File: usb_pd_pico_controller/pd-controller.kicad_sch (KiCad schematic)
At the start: 15 parts, among them J5 USB_C_Receptacle_USB2.0_16P, Q1 STL6P3LLH6, U1 STUSB4531QTR

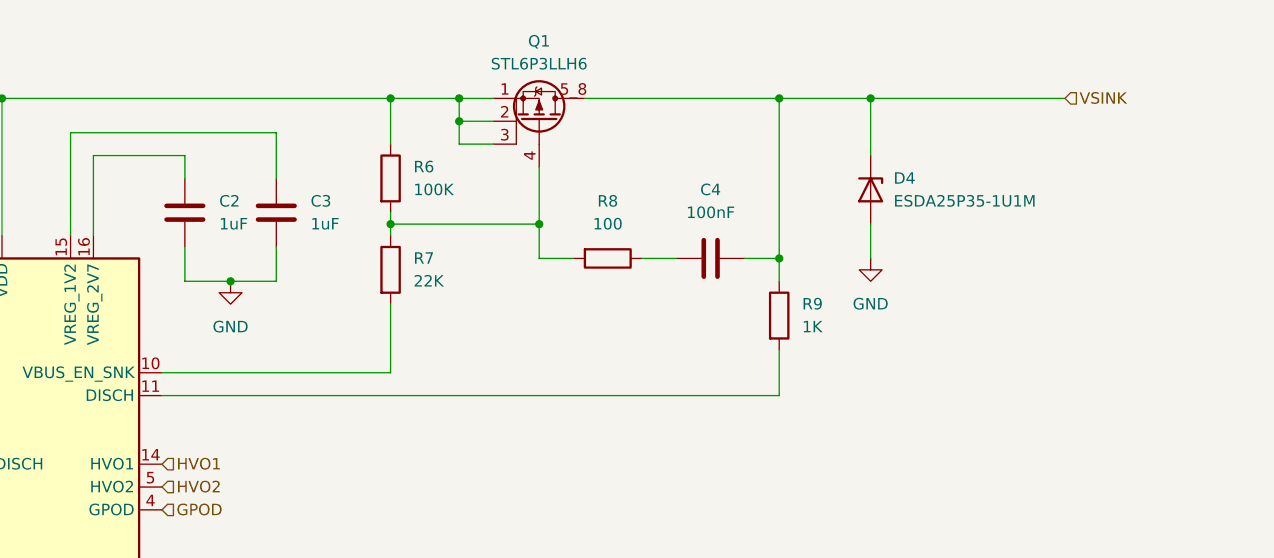
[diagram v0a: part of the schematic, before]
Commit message: Consolidated BOM item (100nF)
Signed-off-by: Thomas Flummer <tf@flummer.net>
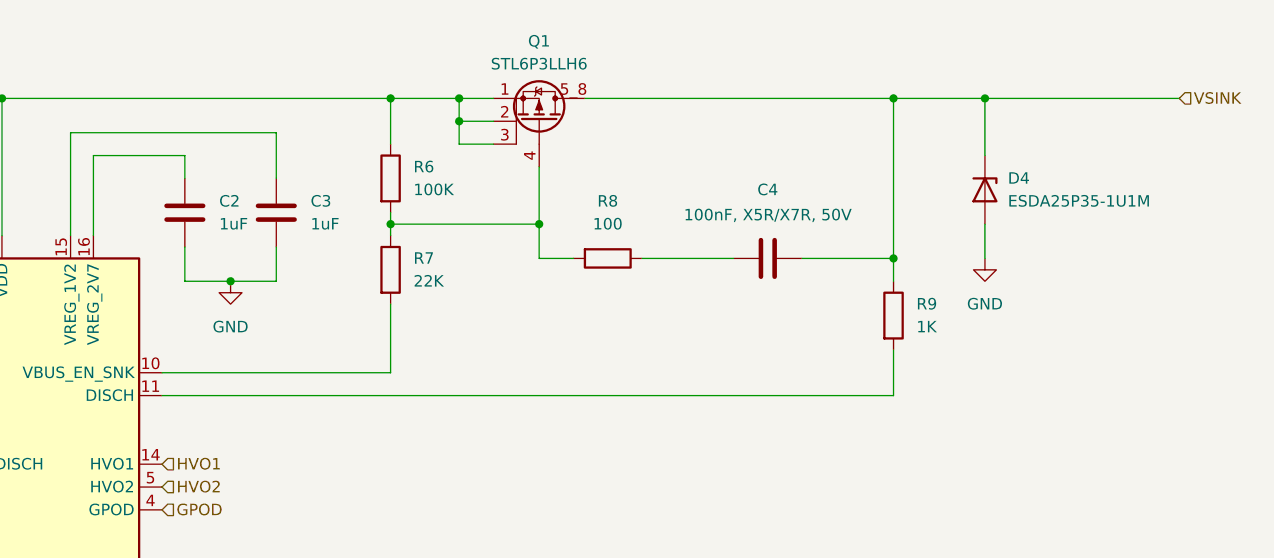
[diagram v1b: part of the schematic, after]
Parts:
- C4: value 100nF -> 100nF, X5R/X7R, 50V
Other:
- moved on the sheet: C4, D4, R9
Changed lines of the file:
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@@
-	)
-	(junction
-		(at 219.71 72.39)
-		(diameter 0)
-		(color 0 0 0 0)
 	)
 	(junction
@@
 	)
 	(junction
-		(at 219.71 54.61)
+		(at 232.41 54.61)
 		(diameter 0)
 		(color 0 0 0 0)
 	)
 	(junction
-		(at 229.87 54.61)
+		(at 242.57 54.61)
 		(diameter 0)
 		(color 0 0 0 0)
@@
 	)
 	(junction
+		(at 232.41 72.39)
+		(diameter 0)
+		(color 0 0 0 0)
+	)
+	(junction
 		(at 97.79 54.61)
 		(diameter 0)
@@
 	(wire
 		(pts
+			(xy 222.25 72.39) (xy 232.41 72.39)
+		)
+		(stroke
+			(width 0)
+			(type default)
+		)
+	)
+	(wire
+		(pts
 			(xy 50.8 54.61) (xy 73.66 54.61)
 		)
@@
 	(wire
 		(pts
-			(xy 198.12 54.61) (xy 219.71 54.61)
-		)
-		(stroke
-			(width 0)
-			(type default)
-		)
-	)
-	(wire
-		(pts
 			(xy 143.51 60.96) (xy 143.51 69.85)
 		)
@@
 	(wire
 		(pts
+			(xy 198.12 54.61) (xy 232.41 54.61)
+		)
+		(stroke
+			(width 0)
+			(type default)
+		)
+	)
+	(wire
+		(pts
 			(xy 68.58 82.55) (xy 68.58 59.69)
 		)
@@
 	(wire
 		(pts
-			(xy 204.47 72.39) (xy 208.28 72.39)
+			(xy 204.47 72.39) (xy 214.63 72.39)
 		)
 		(stroke
@@
 	(wire
 		(pts
-			(xy 219.71 72.39) (xy 219.71 54.61)
+			(xy 232.41 72.39) (xy 232.41 54.61)
 		)
 		(stroke
@@
 	(wire
 		(pts
-			(xy 219.71 82.55) (xy 219.71 87.63)
+			(xy 232.41 82.55) (xy 232.41 87.63)
 		)
 		(stroke
@@
 	(wire
 		(pts
-			(xy 229.87 68.58) (xy 229.87 72.39)
+			(xy 242.57 68.58) (xy 242.57 72.39)
 		)
 		(stroke
@@
 	(wire
 		(pts
-			(xy 215.9 72.39) (xy 219.71 72.39)
-		)
-		(stroke
-			(width 0)
-			(type default)
-		)
-	)
-	(wire
-		(pts
 			(xy 153.67 63.5) (xy 153.67 60.96)
 		)
@@
 	(wire
 		(pts
-			(xy 219.71 54.61) (xy 229.87 54.61)
-		)
-		(stroke
-			(width 0)
-			(type default)
-		)
-	)
-	(wire
-		(pts
-			(xy 219.71 72.39) (xy 219.71 74.93)
-		)
-		(stroke
-			(width 0)
-			(type default)
-		)
-	)
-	(wire
-		(pts
-			(xy 229.87 54.61) (xy 229.87 60.96)
+			(xy 232.41 54.61) (xy 242.57 54.61)
+		)
+		(stroke
+			(width 0)
+			(type default)
+		)
+	)
+	(wire
+		(pts
+			(xy 232.41 72.39) (xy 232.41 74.93)
+		)
+		(stroke
+			(width 0)
+			(type default)
+		)
+	)
+	(wire
+		(pts
+			(xy 151.13 87.63) (xy 232.41 87.63)
+		)
+		(stroke
+			(width 0)
+			(type default)
+		)
+	)
+	(wire
+		(pts
+			(xy 242.57 54.61) (xy 242.57 60.96)
 		)
 		(stroke
@@
 	(wire
 		(pts
-			(xy 219.71 87.63) (xy 151.13 87.63)
-		)
-		(stroke
-			(width 0)
-			(type default)
-		)
-	)
-	(wire
-		(pts
 			(xy 176.53 77.47) (xy 176.53 85.09)
 		)
@@
 	(wire
 		(pts
-			(xy 229.87 54.61) (xy 251.46 54.61)
+			(xy 242.57 54.61) (xy 264.16 54.61)
 		)
 		(stroke
@@
 	(hierarchical_label "VSINK"
 		(shape input)
-		(at 251.46 54.61 0)
+		(at 264.16 54.61 0)
 		(effects
 			(font
@@
 	(symbol
 		(lib_id "power:GND")
-		(at 229.87 72.39 0)
+		(at 242.57 72.39 0)
 		(unit 1)
 		(body_style 1)
@@
 		(fields_autoplaced yes)
 		(property "Reference" "#PWR018"
-			(at 229.87 78.74 0)
+			(at 242.57 78.74 0)
 			(hide yes)
 			(show_name no)
@@
 		)
 		(property "Value" "GND"
-			(at 229.87 77.47 0)
+			(at 242.57 77.47 0)
 			(show_name no)
 			(do_not_autoplace no)
@@
 		)
 		(property "Footprint" ""
-			(at 229.87 72.39 0)
+			(at 242.57 72.39 0)
 			(hide yes)
 			(show_name no)
@@
 		)
 		(property "Datasheet" ""
-			(at 229.87 72.39 0)
+			(at 242.57 72.39 0)
 			(hide yes)
 			(show_name no)
@@
 		)
 		(property "Description" "Power symbol creates a global label with name \"GND\" , ground"
-			(at 229.87 72.39 0)
+			(at 242.57 72.39 0)
 			(hide yes)
 			(show_name no)
@@
 	(symbol
 		(lib_id "Device:C")
-		(at 212.09 72.39 90)
+		(at 218.44 72.39 90)
 		(unit 1)
 		(body_style 1)
@@
 		(in_pos_files yes)
 		(dnp no)
-		(fields_autoplaced yes)
 		(property "Reference" "C4"
-			(at 212.09 64.77 90)
-			(show_name no)
-			(do_not_autoplace no)
-			(effects
-				(font
-					(size 1.27 1.27)
-				)
-			)
-		)
-		(property "Value" "100nF"
-			(at 212.09 67.31 90)
+			(at 218.44 64.77 90)
+			(show_name no)
+			(do_not_autoplace no)
+			(effects
+				(font
+					(size 1.27 1.27)
+				)
+			)
+		)
+		(property "Value" "100nF, X5R/X7R, 50V"
+			(at 218.44 67.564 90)
 			(show_name no)
 			(do_not_autoplace no)
@@
 		)
 		(property "Footprint" "Capacitor_SMD:C_0603_1608Metric"
-			(at 215.9 71.4248 0)
+			(at 222.25 71.4248 0)
 			(hide yes)
 			(show_name no)
@@
 		)
 		(property "Datasheet" ""
-			(at 212.09 72.39 0)
+			(at 218.44 72.39 0)
 			(hide yes)
 			(show_name no)
@@
 		)
 		(property "Description" "Unpolarized capacitor"
-			(at 212.09 72.39 0)
+			(at 218.44 72.39 0)
 			(hide yes)
 			(show_name no)
@@
 	(symbol
 		(lib_id "Device:R")
-		(at 219.71 78.74 0)
+		(at 232.41 78.74 0)
 		(unit 1)
 		(body_style 1)
@@
 		(fields_autoplaced yes)
 		(property "Reference" "R9"
-			(at 222.25 77.4699 0)
+			(at 234.95 77.4699 0)
 			(show_name no)
 			(do_not_autoplace no)
@@
 		)
 		(property "Value" "1K"
-			(at 222.25 80.0099 0)
+			(at 234.95 80.0099 0)
 			(show_name no)
 			(do_not_autoplace no)
@@
 		)
 		(property "Footprint" "Resistor_SMD:R_0603_1608Metric"
-			(at 217.932 78.74 90)
+			(at 230.632 78.74 90)
 			(hide yes)
 			(show_name no)
@@
 		)
 		(property "Datasheet" ""
-			(at 219.71 78.74 0)
+			(at 232.41 78.74 0)
 			(hide yes)
 			(show_name no)
@@
 		)
 		(property "Description" "Resistor"
-			(at 219.71 78.74 0)
+			(at 232.41 78.74 0)
 			(hide yes)
 			(show_name no)
@@
 	(symbol
 		(lib_id "Diode:ESD5Zxx")
-		(at 229.87 64.77 270)
+		(at 242.57 64.77 270)
 		(unit 1)
 		(body_style 1)
@@
 		(fields_autoplaced yes)
 		(property "Reference" "D4"
-			(at 232.41 63.4999 90)
+			(at 245.11 63.4999 90)
 			(show_name no)
 			(do_not_autoplace no)
@@
 		)
 		(property "Value" "ESDA25P35-1U1M"
-			(at 232.41 66.0399 90)
+			(at 245.11 66.0399 90)
 			(show_name no)
 			(do_not_autoplace no)
@@
 		)
 		(property "Footprint" "Diode_SMD:ST_QFN-2L_1.6x1.0mm"
-			(at 225.425 64.77 0)
+			(at 238.125 64.77 0)
 			(hide yes)
 			(show_name no)
@@
 		)
 		(property "Datasheet" "https://www.st.com/resource/en/datasheet/esda25p35-1u1m.pdf"
-			(at 229.87 64.77 0)
+			(at 242.57 64.77 0)
 			(hide yes)
 			(show_name no)
@@
 		)
 		(property "Description" "35 A - 8/20 us, 22 V TVS in QFN-2L"
-			(at 229.87 64.77 0)
-			(hide yes)
-			(show_name no)
+			(at 242.57 64.77 0)
+			(hide yes)
+			(show_name no)
